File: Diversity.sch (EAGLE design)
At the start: 8 parts, among them IC1 LM1881, IC2 LM1881, IC3 MEGA8-AI, IC4 4053N, X1 RCA-4-117-01, X2 RCA-4-117-01

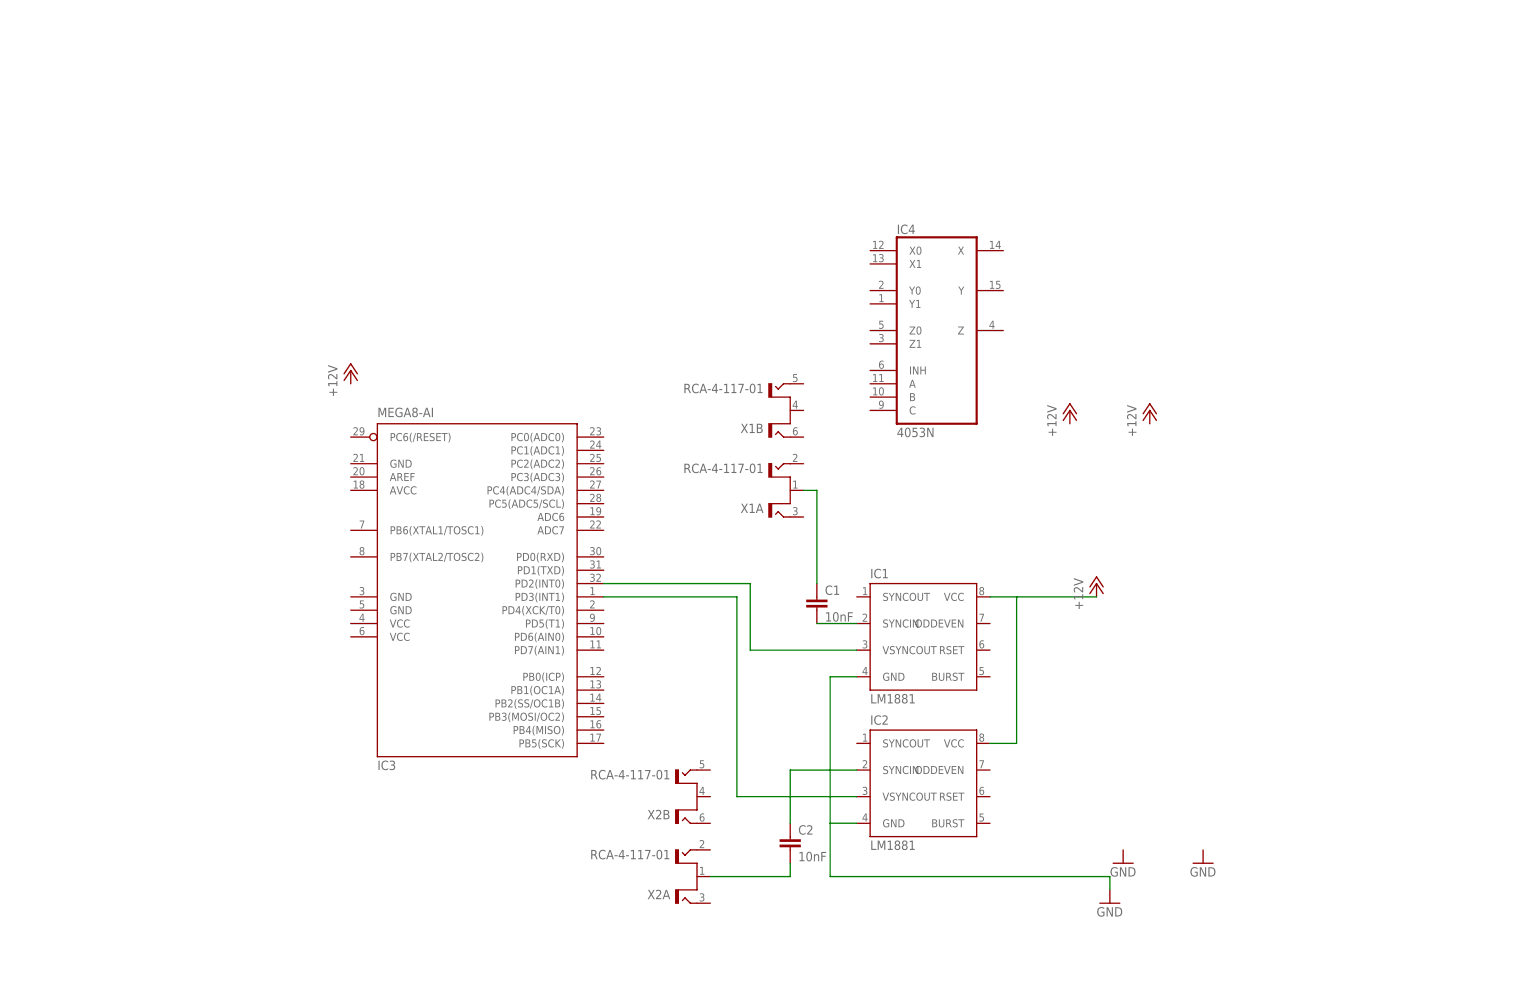
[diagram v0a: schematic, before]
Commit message: asdf
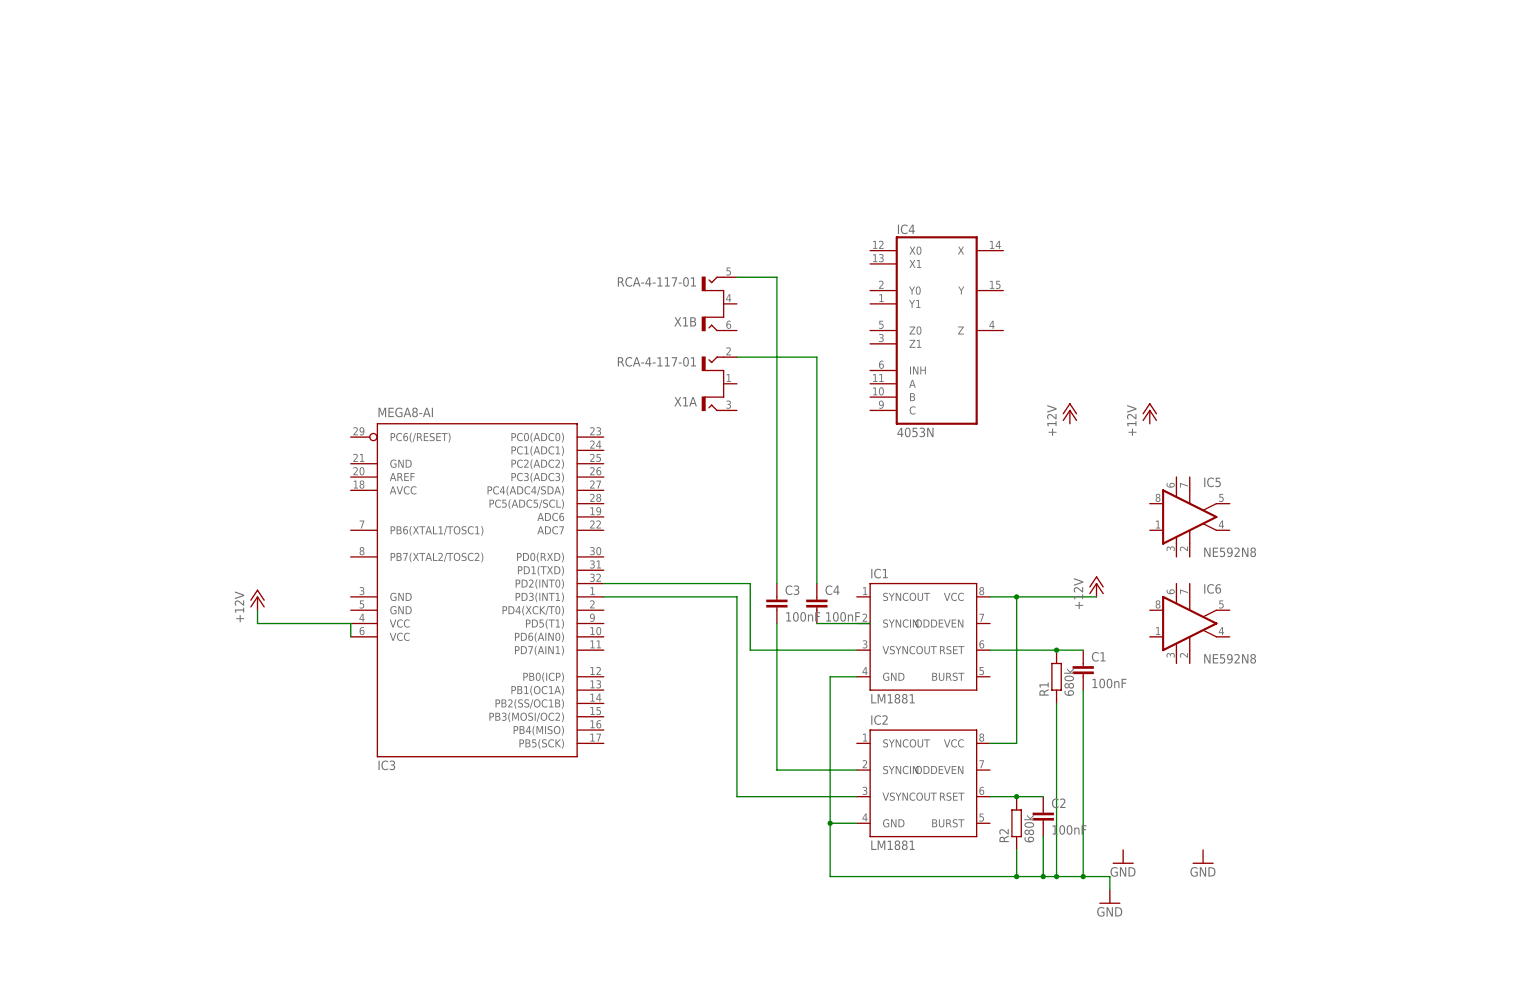
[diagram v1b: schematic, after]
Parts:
- removed X2: RCA-4-117-01, con-conrad:RCA-4-117-01
- added C3, C4: 100nF, capacitor-wima:C2.5/2
- added IC5, IC6: NE592N8, linear:NE592N8
- added R1, R2: 680k, resistor:R-EU_0207/7
- C1, C2: value 10nF -> 100nF; device rcl:C-EU025-024X044 -> capacitor-wima:C2.5/2
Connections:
- removed net N$6: C2.2, X2A.S
- new net N$10: C1.1, IC1.RSET, R1.2
- new net N$7: C3.1, X1B.T1
- new net N$9: C2.1, IC2.RSET, R2.2
- net +12V: now also IC3.VCC@1, IC3.VCC@2
- net GND: now also C1.2, C2.2, R1.1, R2.1
- net N$3: now also C4.1, X1A.T1; no longer C1.1, X1A.S
- net N$4: now also C4.2; no longer C1.2, IC1.SYNCIN
- net N$5: now also C3.2; no longer C2.1
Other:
- moved on the sheet: C1, C2, X1A, X1B
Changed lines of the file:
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@@
 <part name="GND3" library="supply1" deviceset="GND" device=""/>
 <part name="X1" library="con-conrad" deviceset="RCA-4-117-01" device=""/>
-<part name="X2" library="con-conrad" deviceset="RCA-4-117-01" device=""/>
-<part name="C1" library="rcl" deviceset="C-EU" device="025-024X044" value="10nF"/>
-<part name="C2" library="rcl" deviceset="C-EU" device="025-024X044" value="10nF"/>
 <part name="IC4" library="40xx" deviceset="4053" device="N"/>
+<part name="C3" library="capacitor-wima" deviceset="C" device="2.5/2" value="100nF"/>
+<part name="C4" library="capacitor-wima" deviceset="C" device="2.5/2" value="100nF"/>
+<part name="IC5" library="linear" deviceset="NE592?8" device="N"/>
+<part name="IC6" library="linear" deviceset="NE592?8" device="N"/>
+<part name="C1" library="capacitor-wima" deviceset="C" device="2.5/2" value="100nF"/>
+<part name="C2" library="capacitor-wima" deviceset="C" device="2.5/2" value="100nF"/>
+<part name="R1" library="resistor" deviceset="R-EU_" device="0207/7" value="680k"/>
+<part name="R2" library="resistor" deviceset="R-EU_" device="0207/7" value="680k"/>
 </parts>
 <sheets>
@@
 <instance part="IC2" gate="G$1" x="104.14" y="17.78"/>
 <instance part="IC3" gate="G$1" x="17.78" y="58.42"/>
-<instance part="P+1" gate="1" x="-5.08" y="96.52"/>
+<instance part="P+1" gate="1" x="-22.86" y="53.34"/>
 <instance part="P+2" gate="1" x="137.16" y="55.88"/>
 <instance part="P+3" gate="1" x="132.08" y="88.9"/>
@@
 <instance part="GND2" gate="1" x="142.24" y="2.54"/>
 <instance part="GND3" gate="1" x="157.48" y="2.54"/>
-<instance part="X1" gate="A" x="76.2" y="73.66" rot="R180"/>
-<instance part="X1" gate="B" x="76.2" y="88.9" rot="R180"/>
-<instance part="X2" gate="A" x="58.42" y="0" rot="R180"/>
-<instance part="X2" gate="B" x="58.42" y="15.24" rot="R180"/>
-<instance part="C1" gate="G$1" x="83.82" y="53.34"/>
-<instance part="C2" gate="G$1" x="78.74" y="7.62"/>
+<instance part="X1" gate="A" x="63.5" y="93.98" rot="R180"/>
+<instance part="X1" gate="B" x="63.5" y="109.22" rot="R180"/>
 <instance part="IC4" gate="A" x="106.68" y="104.14"/>
+<instance part="C3" gate="G$1" x="76.2" y="53.34"/>
+<instance part="C4" gate="G$1" x="83.82" y="53.34"/>
+<instance part="IC5" gate="A" x="154.94" y="68.58"/>
+<instance part="IC6" gate="A" x="154.94" y="48.26"/>
+<instance part="C1" gate="G$1" x="134.62" y="40.64"/>
+<instance part="C2" gate="G$1" x="127" y="12.7"/>
+<instance part="R1" gate="G$1" x="129.54" y="38.1" rot="R90"/>
+<instance part="R2" gate="G$1" x="121.92" y="10.16" rot="R90"/>
 </instances>
 <busses>
@@
 <wire x1="116.84" y1="25.4" x2="121.92" y2="25.4" width="0.1524" layer="91"/>
 <wire x1="121.92" y1="25.4" x2="121.92" y2="53.34" width="0.1524" layer="91"/>
+<junction x="121.92" y="53.34"/>
+</segment>
+<segment>
+<pinref part="IC3" gate="G$1" pin="VCC@2"/>
+<pinref part="IC3" gate="G$1" pin="VCC@1"/>
+<wire x1="-5.08" y1="45.72" x2="-5.08" y2="48.26" width="0.1524" layer="91"/>
+<wire x1="-5.08" y1="48.26" x2="-22.86" y2="48.26" width="0.1524" layer="91"/>
+<pinref part="P+1" gate="1" pin="+12V"/>
+<wire x1="-22.86" y1="48.26" x2="-22.86" y2="50.8" width="0.1524" layer="91"/>
 </segment>
 </net>
@@
 <wire x1="86.36" y1="10.16" x2="86.36" y2="0" width="0.1524" layer="91"/>
 <pinref part="GND1" gate="1" pin="GND"/>
-<wire x1="86.36" y1="0" x2="139.7" y2="0" width="0.1524" layer="91"/>
+<wire x1="86.36" y1="0" x2="121.92" y2="0" width="0.1524" layer="91"/>
+<wire x1="121.92" y1="0" x2="127" y2="0" width="0.1524" layer="91"/>
+<wire x1="134.62" y1="0" x2="139.7" y2="0" width="0.1524" layer="91"/>
 <wire x1="139.7" y1="0" x2="139.7" y2="-2.54" width="0.1524" layer="91"/>
 <pinref part="IC1" gate="G$1" pin="GND"/>
 <wire x1="91.44" y1="38.1" x2="86.36" y2="38.1" width="0.1524" layer="91"/>
 <wire x1="86.36" y1="38.1" x2="86.36" y2="10.16" width="0.1524" layer="91"/>
+<junction x="86.36" y="10.16"/>
+<pinref part="C2" gate="G$1" pin="2"/>
+<wire x1="127" y1="7.62" x2="127" y2="0" width="0.1524" layer="91"/>
+<pinref part="C1" gate="G$1" pin="2"/>
+<wire x1="127" y1="0" x2="129.54" y2="0" width="0.1524" layer="91"/>
+<wire x1="129.54" y1="0" x2="134.62" y2="0" width="0.1524" layer="91"/>
+<wire x1="134.62" y1="0" x2="134.62" y2="35.56" width="0.1524" layer="91"/>
+<pinref part="R2" gate="G$1" pin="1"/>
+<wire x1="121.92" y1="5.08" x2="121.92" y2="0" width="0.1524" layer="91"/>
+<pinref part="R1" gate="G$1" pin="1"/>
+<wire x1="129.54" y1="33.02" x2="129.54" y2="0" width="0.1524" layer="91"/>
+<junction x="121.92" y="0"/>
+<junction x="127" y="0"/>
+<junction x="129.54" y="0"/>
+<junction x="134.62" y="0"/>
+</segment>
+</net>
+<net name="N$5" class="0">
+<segment>
+<pinref part="IC2" gate="G$1" pin="SYNCIN"/>
+<wire x1="76.2" y1="20.32" x2="91.44" y2="20.32" width="0.1524" layer="91"/>
+<pinref part="C3" gate="G$1" pin="2"/>
+<wire x1="76.2" y1="48.26" x2="76.2" y2="20.32" width="0.1524" layer="91"/>
 </segment>
 </net>
 <net name="N$3" class="0">
 <segment>
-<pinref part="X1" gate="A" pin="S"/>
-<wire x1="81.28" y1="73.66" x2="83.82" y2="73.66" width="0.1524" layer="91"/>
-<wire x1="83.82" y1="73.66" x2="83.82" y2="55.88" width="0.1524" layer="91"/>
-<pinref part="C1" gate="G$1" pin="1"/>
+<pinref part="X1" gate="A" pin="T1"/>
+<wire x1="68.58" y1="99.06" x2="83.82" y2="99.06" width="0.1524" layer="91"/>
+<wire x1="83.82" y1="99.06" x2="83.82" y2="55.88" width="0.1524" layer="91"/>
+<pinref part="C4" gate="G$1" pin="1"/>
 </segment>
 </net>
 <net name="N$4" class="0">
 <segment>
-<pinref part="C1" gate="G$1" pin="2"/>
-<pinref part="IC1" gate="G$1" pin="SYNCIN"/>
-<wire x1="83.82" y1="48.26" x2="91.44" y2="48.26" width="0.1524" layer="91"/>
+<pinref part="C4" gate="G$1" pin="2"/>
+<wire x1="83.82" y1="48.26" x2="93.98" y2="48.26" width="0.1524" layer="91"/>
 </segment>
 </net>
-<net name="N$5" class="0">
+<net name="N$7" class="0">
+<segment>
+<pinref part="C3" gate="G$1" pin="1"/>
+<wire x1="76.2" y1="55.88" x2="76.2" y2="114.3" width="0.1524" layer="91"/>
+<pinref part="X1" gate="B" pin="T1"/>
+<wire x1="76.2" y1="114.3" x2="68.58" y2="114.3" width="0.1524" layer="91"/>
+</segment>
+</net>
+<net name="N$9" class="0">
 <segment>
 <pinref part="C2" gate="G$1" pin="1"/>
-<wire x1="78.74" y1="10.16" x2="78.74" y2="20.32" width="0.1524" layer="91"/>
-<pinref part="IC2" gate="G$1" pin="SYNCIN"/>
-<wire x1="78.74" y1="20.32" x2="91.44" y2="20.32" width="0.1524" layer="91"/>
+<pinref part="IC2" gate="G$1" pin="RSET"/>
+<wire x1="127" y1="15.24" x2="121.92" y2="15.24" width="0.1524" layer="91"/>
+<pinref part="R2" gate="G$1" pin="2"/>
+<wire x1="121.92" y1="15.24" x2="116.84" y2="15.24" width="0.1524" layer="91"/>
+<junction x="121.92" y="15.24"/>
 </segment>
 </net>
-<net name="N$6" class="0">
+<net name="N$10" class="0">
 <segment>
-<pinref part="X2" gate="A" pin="S"/>
-<wire x1="63.5" y1="0" x2="78.74" y2="0" width="0.1524" layer="91"/>
-<pinref part="C2" gate="G$1" pin="2"/>
-<wire x1="78.74" y1="0" x2="78.74" y2="2.54" width="0.1524" layer="91"/>
+<pinref part="C1" gate="G$1" pin="1"/>
+<pinref part="IC1" gate="G$1" pin="RSET"/>
+<wire x1="134.62" y1="43.18" x2="129.54" y2="43.18" width="0.1524" layer="91"/>
+<pinref part="R1" gate="G$1" pin="2"/>
+<wire x1="129.54" y1="43.18" x2="116.84" y2="43.18" width="0.1524" layer="91"/>
+<junction x="129.54" y="43.18"/>
 </segment>
 </net>

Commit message: nächster Schritt
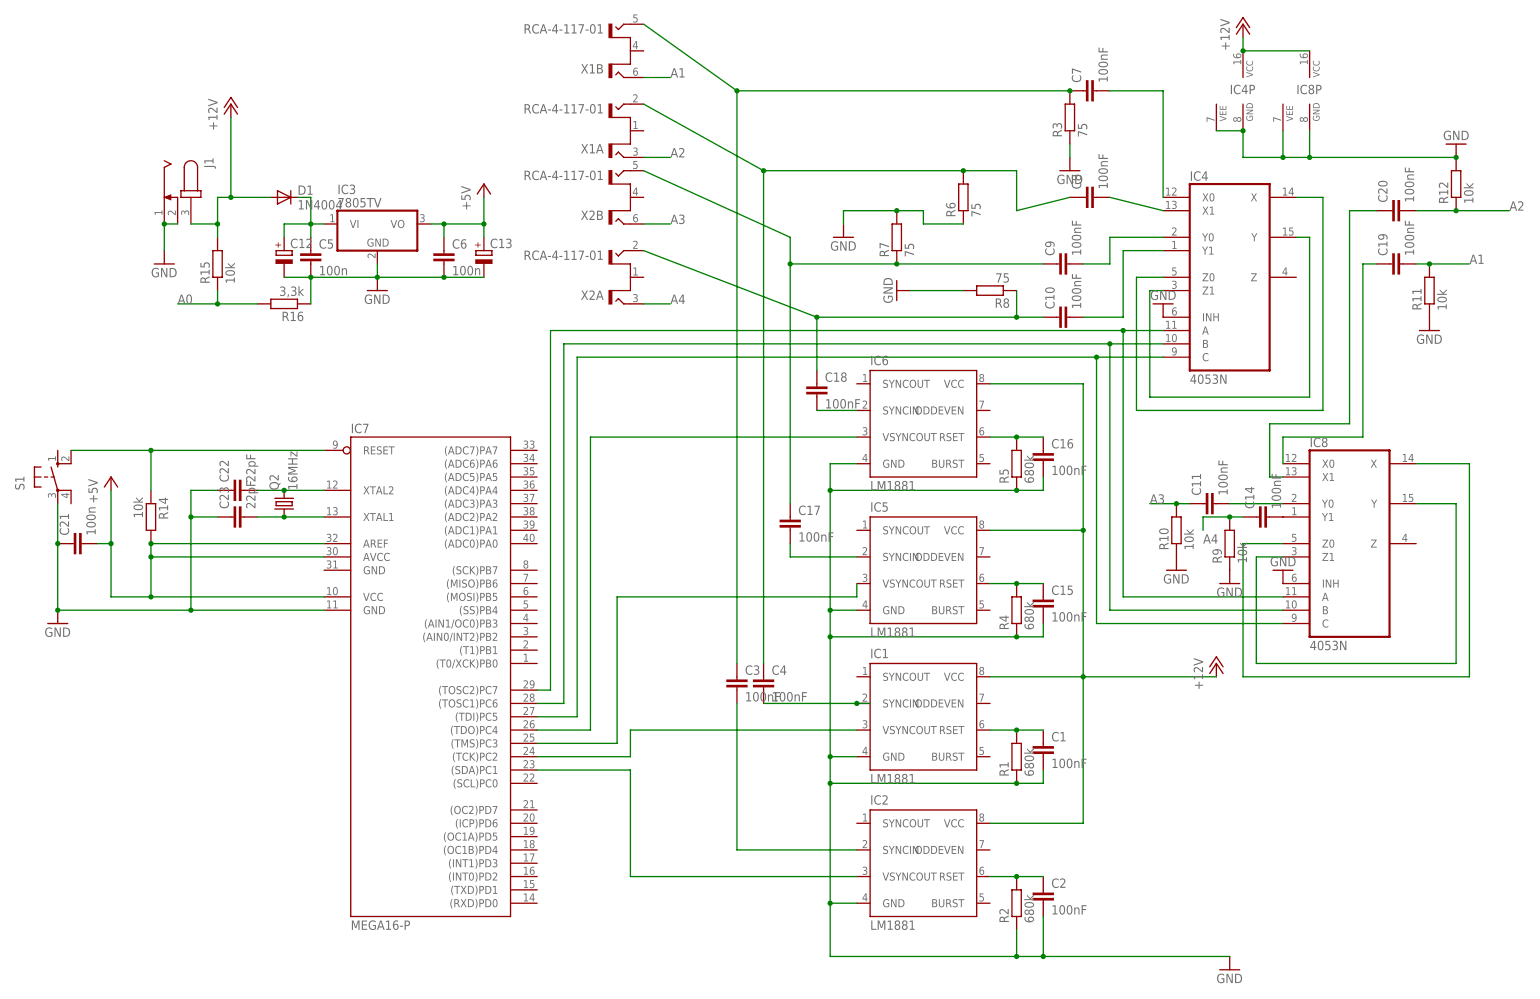
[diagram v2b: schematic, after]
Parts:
- added C10, C11, C14, C15, C16, C17, C18, C19, C20, C7, C8, C9: 100nF, capacitor-wima:C2.5/2
- added C12: (no value), rcl:CPOL-EUE3.5-8
- added C13: (no value), rcl:CPOL-EUE2.5-5
- added C21, C5, C6: 100n, rcl:C-EUC0805
- added C22, C23: 22pF, rcl:C-EUC0805
- added D1: 1N4004, diode:1N4004
- added IC7: MEGA16-P, atmel:MEGA16-P
- added IC8: 4053N, 40xx:4053N
- added J1: (no value), con-jack:JACK-PLUG0
- added Q2: 16MHz, crystal:CRYSTALSM49
- added R10, R11, R12, R14, R9: 10k, resistor:R-EU_0207/7
- added R15: 10k, rcl:R-EU_R0805
- added R16: 3,3k, rcl:R-EU_R0805
- added R3, R6, R7, R8: 75, resistor:R-EU_0207/7
- added R4, R5: 680k, resistor:R-EU_0207/7
- added S1: (no value), switch-omron:10-XX
- added X2: RCA-4-117-01, con-conrad:RCA-4-117-01
- IC3: value MEGA8-AI -> 7805TV; device atmel:MEGA8-AI -> linear:7805TV
- IC5, IC6: value NE592N8 -> LM1881; device linear:NE592N8 -> lm1881:LM1881
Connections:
- new net +5V: C13.+, C21.2, C6.1, IC3.VO, IC7.AREF, IC7.AVCC, IC7.VCC, R14.2
- new net A0: R15.1, R16.2
- new net A1: C19.2, R11.2, X1B.T2
- new net A2: C20.2, R12.1, X1A.T2
- new net A3: C11.1, R10.2, X2B.T2
- new net A4: C14.1, R9.2, X2A.T2
- new net N$11: C8.2, IC4A.X1
- new net N$12: C9.2, IC4A.Y0
- new net N$13: C10.2, IC4A.Y1
- new net N$14: IC5.VSYNCOUT, IC7.(TMS)PC3
- new net N$15: IC6.VSYNCOUT, IC7.(TDO)PC4
- new net N$16: C14.2, IC8A.Y1
- new net N$17: C16.1, IC6.RSET, R5.2
- new net N$18: C15.1, IC5.RSET, R4.2
- new net N$19: C17.2, IC5.SYNCIN
- new net N$20: C17.1, C9.1, R7.1, X2B.T1
- new net N$21: IC4A.C, IC7.(TDI)PC5, IC8A.C
- new net N$22: C18.2, IC6.SYNCIN
- new net N$23: C10.1, C18.1, R8.1, X2A.T1
- new net N$24: IC4A.X, IC4A.Z0
- new net N$25: IC4A.Y, IC4A.Z1
- new net N$26: IC4A.B, IC7.(TOSC1)PC6, IC8A.B
- new net N$27: IC4A.A, IC7.(TOSC2)PC7, IC8A.A
- new net N$28: C11.2, IC8A.Y0
- new net N$29: C19.1, IC8A.X0
- new net N$30: C20.1, IC8A.X1
- new net N$31: IC8A.X, IC8A.Z0
- new net N$32: IC8A.Y, IC8A.Z1
- new net N$33: IC7.RESET, R14.1, S1.S1
- new net N$34: C23.2, IC7.XTAL1, Q2.1
- new net N$35: C22.2, IC7.XTAL2, Q2.2
- new net N$6: C7.2, IC4A.X0
- new net N$8: C12.+, C5.1, D1.C, IC3.VI
- net +12V: now also D1.A, IC4P.VCC, IC5.VCC, IC6.VCC, IC8P.VCC, J1.3, R15.2; no longer IC3.VCC@1, IC3.VCC@2
- net GND: now also C12.-, C13.-, C15.2, C16.2, C21.1, C22.1, C23.1, C5.2, C6.2, IC3.GND, IC4A.INH, IC4P.GND, IC4P.VEE, IC5.GND, IC6.GND, IC7.GND, IC8A.INH, IC8P.GND, IC8P.VEE, J1.1, J1.2, R10.1, R11.1, R12.2, R16.1, R3.1, R4.1, R5.1, R6.1, R7.2, R8.2, R9.1, S1.P
- net N$1: now also IC7.(TCK)PC2; no longer IC3.PD2(INT0)
- net N$2: now also IC7.(SDA)PC1; no longer IC3.PD3(INT1)
- net N$3: now also C8.1, R6.2
- net N$4: now also IC1.SYNCIN
- net N$7: now also C7.1, R3.2
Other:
- moved on the sheet: C1, C2, C3, C4, IC1, IC2, IC4, R1, R2, X1A, X1B
